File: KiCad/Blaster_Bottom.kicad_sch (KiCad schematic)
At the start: 24 parts, among them J2 Power & Output Test Points, J3 Inputs Test Points, Q1 BUK9832-55A, Q2 BUK9832-55A, Q3 BUK9832-55A, U2 PIC16F1788-IP

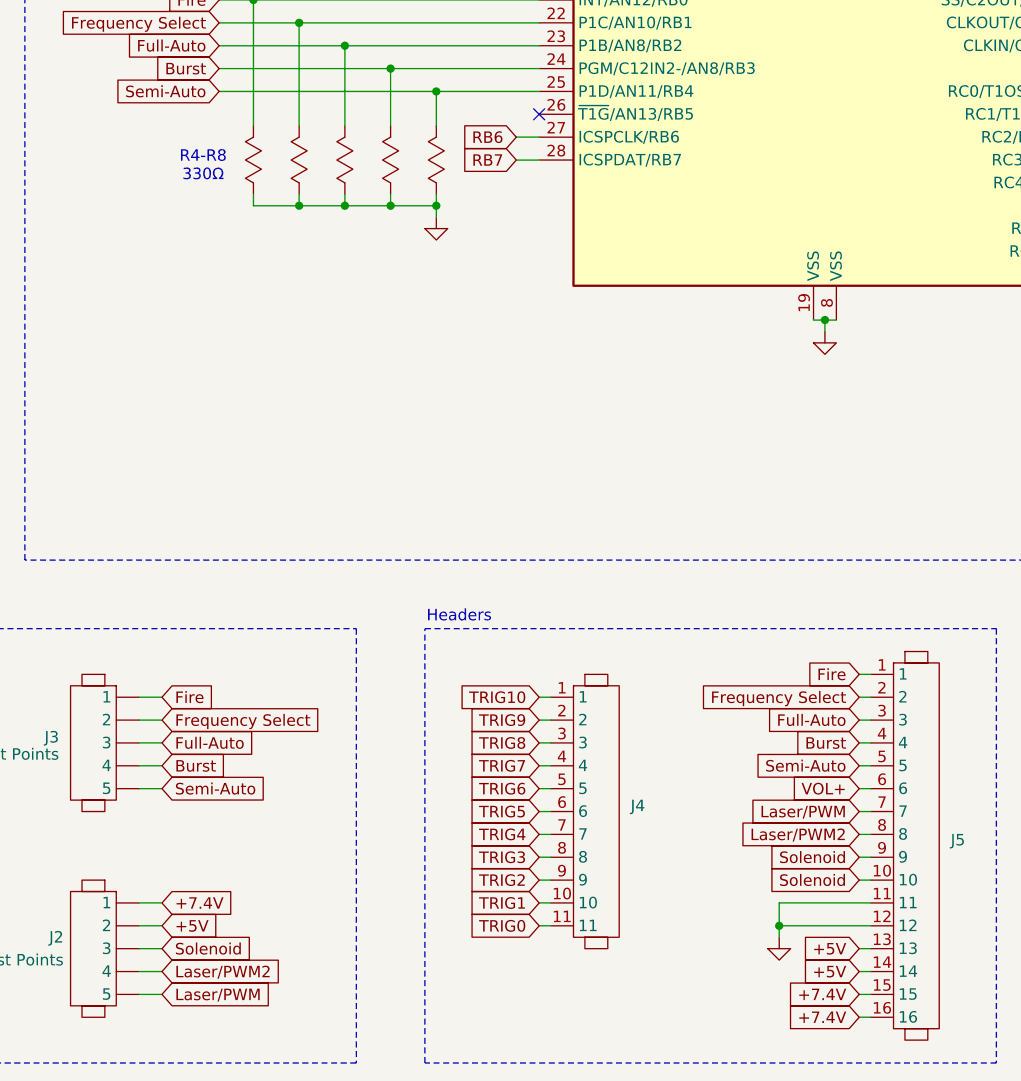
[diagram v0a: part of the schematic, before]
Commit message: updated blaster schematic
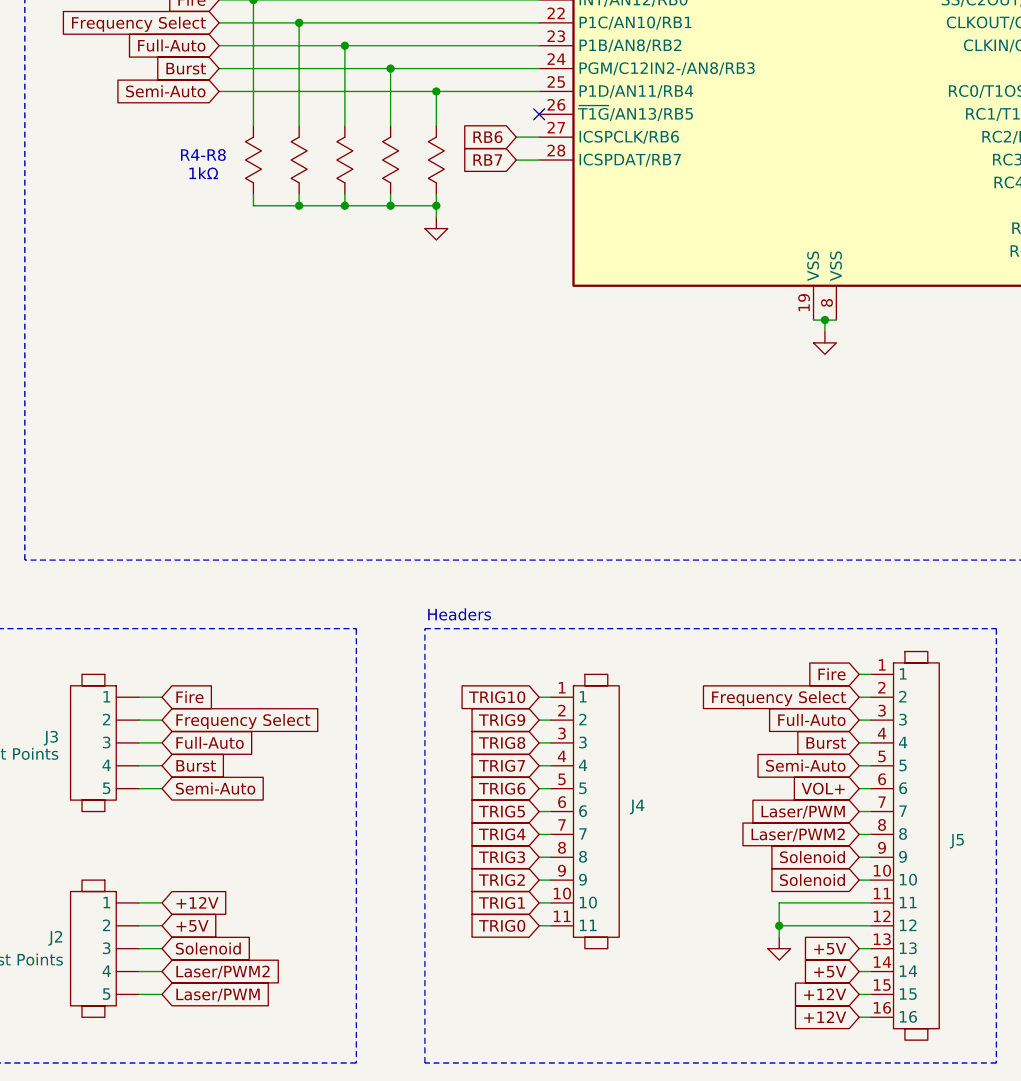
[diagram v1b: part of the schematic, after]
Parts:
- R4, R5, R6, R7, R8: value 330Ω -> 1kΩ
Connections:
- net +7.4V renamed +12V
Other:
- note added: "R4-R8 1kΩ"
- note removed: "R4-R8 330Ω"
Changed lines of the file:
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@@
 		)
 	)
-	(text "R4-R8\n330Ω"
+	(text "R4-R8\n1kΩ"
 		(exclude_from_sim no)
 		(at 65.532 98.552 0)
@@
 		)
 	)
-	(global_label "+7.4V"
+	(global_label "+12V"
 		(shape input)
 		(at 60.96 180.34 0)
@@
 		)
 		(property "Intersheetrefs" "${INTERSHEET_REFS}"
-			(at 69.63 180.34 0)
+			(at 69.0252 180.34 0)
 			(effects
 				(font
@@
 		)
 	)
-	(global_label "+7.4V"
+	(global_label "+12V"
 		(shape input)
 		(at 138.43 193.04 180)
@@
 		)
 		(property "Intersheetrefs" "${INTERSHEET_REFS}"
-			(at 129.76 193.04 0)
+			(at 130.3648 193.04 0)
 			(effects
 				(font
@@
 		)
 	)
-	(global_label "+7.4V"
+	(global_label "+12V"
 		(shape input)
 		(at 138.43 190.5 180)
@@
 		)
 		(property "Intersheetrefs" "${INTERSHEET_REFS}"
-			(at 129.76 190.5 0)
+			(at 130.3648 190.5 0)
 			(effects
 				(font
@@
 			)
 		)
-		(property "Value" "330Ω"
+		(property "Value" "1kΩ"
 			(at 80.01 99.06 90)
 			(effects
@@
 			)
 		)
-		(property "Value" "330Ω"
+		(property "Value" "1kΩ"
 			(at 68.58 98.806 90)
 			(effects
@@
 			)
 		)
-		(property "Value" "330Ω"
+		(property "Value" "1kΩ"
 			(at 74.93 99.06 90)
 			(effects
@@
 			)
 		)
-		(property "Value" "330Ω"
+		(property "Value" "1kΩ"
 			(at 85.09 99.06 90)
 			(effects
@@
 			)
 		)
-		(property "Value" "330Ω"
+		(property "Value" "1kΩ"
 			(at 90.17 99.06 90)
 			(effects
